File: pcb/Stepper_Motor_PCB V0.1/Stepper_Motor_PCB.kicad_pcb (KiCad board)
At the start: 2 copper layers, 67 x 50.9 mm, 29 parts, among them J1 Pwr/Coms, J2 Pot, J3 Bootloader Pins, J4 Stepper_Motor, J5 LED, J7 8P8C, SW1 SW_Push, U1 ATmega328P-AU, Y1 Crystal

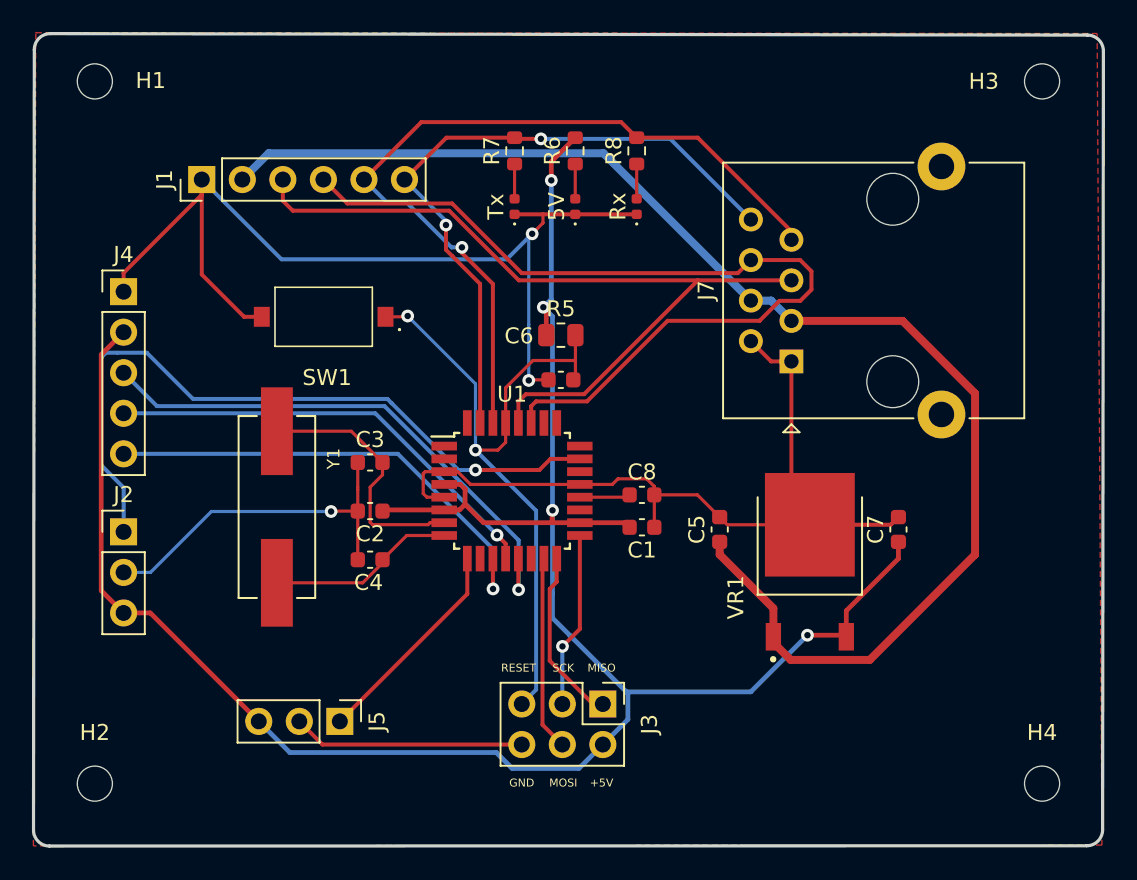
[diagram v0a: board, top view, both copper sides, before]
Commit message: update pcb
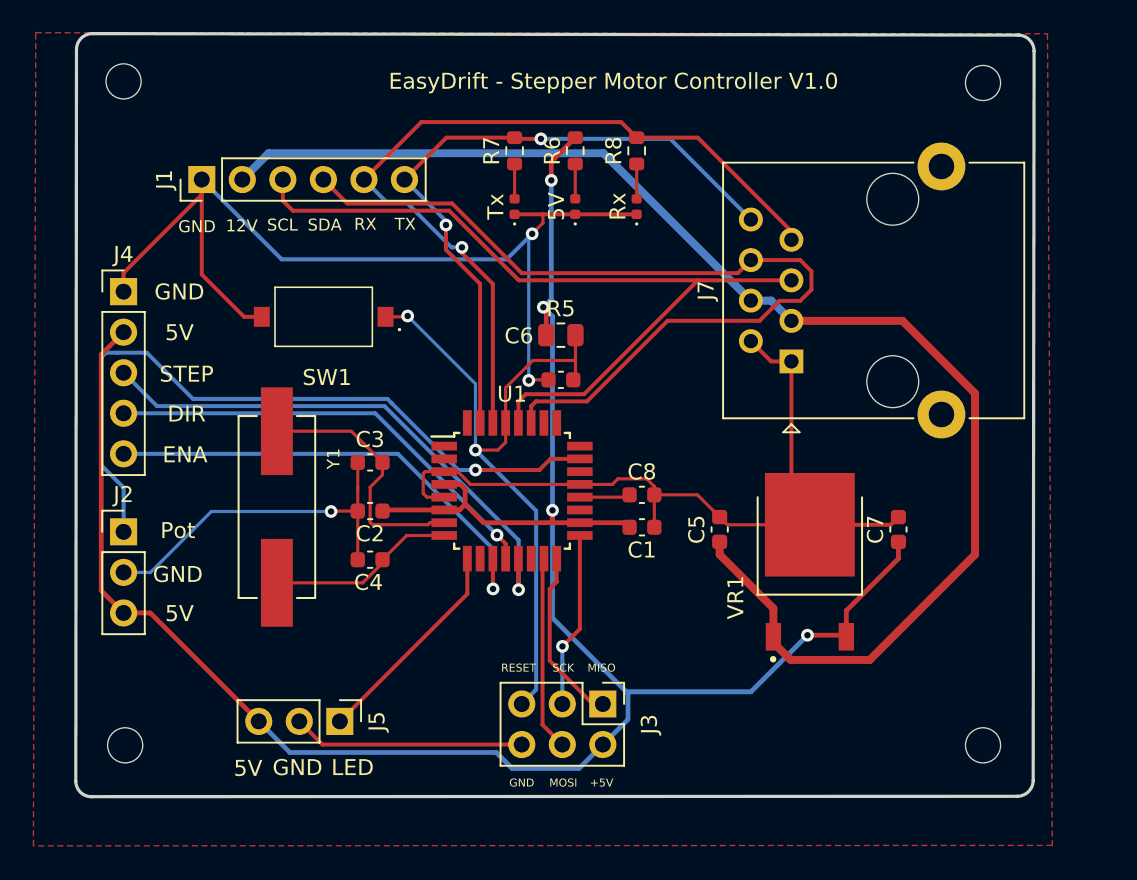
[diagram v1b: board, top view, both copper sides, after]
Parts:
- moved H4 4.41 mm to (178.8, 114.5)
- moved H3 3.70 mm to (178.8, 73.0)
- moved H2 3.06 mm to (125.1, 114.5)
- moved H1 1.80 mm to (125.0, 72.9)
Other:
- board size 67 x 50.9 mm -> 60 x 47.8 mm
- board text added: "12V"
- board text added: "5V"
- board text added: "DIR"
- board text added: "ENA"
- board text added: "EasyDrift - Stepper Motor Controller V1.0"
- board text added: "LED"
- board text added: "Pot"
- board text added: "RX"
- board text added: "SCL"
- board text added: "SDA"
- board text added: "STEP"
- board text added: "TX"
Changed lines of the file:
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@@
   )
   (footprint "MountingHole:MountingHole_2.2mm_M2" (layer "F.Cu")
-    (at 123.2 116.9)
+    (at 125.1 114.5)
     (descr "Mounting Hole 2.2mm, no annular, M2")
     (tags "mounting hole 2.2mm no annular m2")
@@
     (property "Sheetname" "")
     (attr exclude_from_pos_files)
-    (fp_text reference "H2" (at 0 -3.2) (layer "F.SilkS")
+    (fp_text reference "H2" (at 0 -3.2) (layer "F.SilkS") hide
       (effects (font (size 1 1) (thickness 0.15)))
     )
@@
   )
   (footprint "MountingHole:MountingHole_2.2mm_M2" (layer "F.Cu")
-    (at 182.55 72.9)
+    (at 178.85 73)
     (descr "Mounting Hole 2.2mm, no annular, M2")
     (tags "mounting hole 2.2mm no annular m2")
@@
     (property "Sheetname" "")
     (attr exclude_from_pos_files)
-    (fp_text reference "H3" (at -3.65 0) (layer "F.SilkS")
+    (fp_text reference "H3" (at -3.65 0) (layer "F.SilkS") hide
       (effects (font (size 1 1) (thickness 0.15)))
     )
@@
   )
   (footprint "MountingHole:MountingHole_2.2mm_M2" (layer "F.Cu")
-    (at 182.55 116.9)
+    (at 178.85 114.5)
     (descr "Mounting Hole 2.2mm, no annular, M2")
     (tags "mounting hole 2.2mm no annular m2")
@@
     (property "Sheetname" "")
     (attr exclude_from_pos_files)
-    (fp_text reference "H4" (at 0 -3.2) (layer "F.SilkS")
+    (fp_text reference "H4" (at 0 -3.2) (layer "F.SilkS") hide
       (effects (font (size 1 1) (thickness 0.15)))
     )
@@
   )
   (footprint "MountingHole:MountingHole_2.2mm_M2" (layer "F.Cu")
-    (at 123.2 72.9)
+    (at 125 72.9)
     (descr "Mounting Hole 2.2mm, no annular, M2")
     (tags "mounting hole 2.2mm no annular m2")
@@
     (property "Sheetname" "")
     (attr exclude_from_pos_files)
-    (fp_text reference "H1" (at 3.5 -0.05) (layer "F.SilkS")
+    (fp_text reference "H1" (at 3.5 -0.05) (layer "F.SilkS") hide
       (effects (font (size 1 1) (thickness 0.15)))
     )
@@
     )
   )
-  (gr_line (start 185.342893 120.792893) (end 120.357107 120.810661) (layer "Edge.Cuts") (width 0.2))
-  (gr_line (start 119.357107 119.810661) (end 119.407107 70.907107) (layer "Edge.Cuts") (width 0.2))
-  (gr_arc (start 185.392893 70) (mid 186.1 70.292893) (end 186.392893 71) (layer "Edge.Cuts") (width 0.2))
-  (gr_arc (start 119.407107 70.907107) (mid 119.700001 70.200003) (end 120.407107 69.907107) (layer "Edge.Cuts") (width 0.2))
-  (gr_line (start 186.392893 71) (end 186.342893 119.792893) (layer "Edge.Cuts") (width 0.2))
-  (gr_line (start 120.407107 69.907107) (end 185.392893 70) (layer "Edge.Cuts") (width 0.2))
-  (gr_arc (start 120.357107 120.810661) (mid 119.649996 120.51777) (end 119.357107 119.810661) (layer "Edge.Cuts") (width 0.2))
-  (gr_arc (start 186.342893 119.792893) (mid 186.05 120.5) (end 185.342893 120.792893) (layer "Edge.Cuts") (width 0.2))
-  (gr_rect (start 128.257 83.312) (end 160.261 108.966) (layer "User.1") (width 0.5) (fill none))
+  (gr_line (start 180.992893 117.692891) (end 123.007111 117.717768) (layer "Edge.Cuts") (width 0.2))
+  (gr_line (start 122.007111 116.742893) (end 122.05 70.907107) (layer "Edge.Cuts") (width 0.2))
+  (gr_arc (start 181.05 70) (mid 181.757111 70.292891) (end 182.05 71) (layer "Edge.Cuts") (width 0.2))
+  (gr_arc (start 122.05 70.907107) (mid 122.342891 70.199998) (end 123.05 69.907107) (layer "Edge.Cuts") (width 0.2))
+  (gr_line (start 182.05 71) (end 181.992893 116.692891) (layer "Edge.Cuts") (width 0.2))
+  (gr_line (start 123.05 69.907107) (end 181.05 70) (layer "Edge.Cuts") (width 0.2))
+  (gr_arc (start 123.007111 117.717768) (mid 122.301554 117.441185) (end 122.007111 116.742893) (layer "Edge.Cuts") (width 0.2))
+  (gr_arc (start 181.992893 116.692891) (mid 181.700002 117.4) (end 180.992893 117.692891) (layer "Edge.Cuts") (width 0.2))
   (gr_text "MOSI" (at 152.55 116.85) (layer "F.SilkS")
     (effects (font (size 0.5 0.5) (thickness 0.125)))
   )
+  (gr_text "ENA" (at 128.85 96.3) (layer "F.SilkS")
+    (effects (font (size 1 1) (thickness 0.15)))
+  )
+  (gr_text "GND" (at 128.5 86.1) (layer "F.SilkS")
+    (effects (font (size 1 1) (thickness 0.15)))
+  )
   (gr_text "RESET" (at 149.75 109.65) (layer "F.SilkS")
     (effects (font (size 0.5 0.5) (thickness 0.125)))
   )
+  (gr_text "STEP" (at 128.95 91.25) (layer "F.SilkS")
+    (effects (font (size 1 1) (thickness 0.15)))
+  )
   (gr_text "MISO" (at 154.95 109.65) (layer "F.SilkS")
     (effects (font (size 0.5 0.5) (thickness 0.125)))
   )
+  (gr_text "Pot" (at 128.4 101.05) (layer "F.SilkS")
+    (effects (font (size 1 1) (thickness 0.15)))
+  )
+  (gr_text "SDA" (at 137.6 81.9) (layer "F.SilkS")
+    (effects (font (size 0.75 0.75) (thickness 0.15)))
+  )
+  (gr_text "GND" (at 135.9 115.9) (layer "F.SilkS")
+    (effects (font (size 1 1) (thickness 0.15)))
+  )
+  (gr_text "GND" (at 128.4 103.8) (layer "F.SilkS")
+    (effects (font (size 1 1) (thickness 0.15)))
+  )
+  (gr_text "SCL" (at 134.95 81.9) (layer "F.SilkS")
+    (effects (font (size 0.75 0.75) (thickness 0.15)))
+  )
+  (gr_text "EasyDrift - Stepper Motor Controller V1.0" (at 155.7 72.9) (layer "F.SilkS")
+    (effects (font (size 1 1) (thickness 0.15)))
+  )
+  (gr_text "5V" (at 132.8 115.95) (layer "F.SilkS")
+    (effects (font (size 1 1) (thickness 0.15)))
+  )
+  (gr_text "LED" (at 139.35 115.9) (layer "F.SilkS")
+    (effects (font (size 1 1) (thickness 0.15)))
+  )
+  (gr_text "5V" (at 128.5 106.25) (layer "F.SilkS")
+    (effects (font (size 1 1) (thickness 0.15)))
+  )
+  (gr_text "TX" (at 142.65 81.85) (layer "F.SilkS")
+    (effects (font (size 0.75 0.75) (thickness 0.15)))
+  )
+  (gr_text "DIR" (at 128.95 93.75) (layer "F.SilkS")
+    (effects (font (size 1 1) (thickness 0.15)))
+  )
+  (gr_text "12V" (at 132.4 81.95) (layer "F.SilkS")
+    (effects (font (size 0.75 0.75) (thickness 0.15)))
+  )
   (gr_text "SCK" (at 152.55 109.65) (layer "F.SilkS")
     (effects (font (size 0.5 0.5) (thickness 0.125)))
   )
+  (gr_text "5V" (at 128.5 88.65) (layer "F.SilkS")
+    (effects (font (size 1 1) (thickness 0.15)))
+  )
   (gr_text "+5V" (at 154.95 116.85) (layer "F.SilkS")
     (effects (font (size 0.5 0.5) (thickness 0.125)))
+  )
+  (gr_text "GND" (at 129.6 82) (layer "F.SilkS")
+    (effects (font (size 0.75 0.75) (thickness 0.15)))
+  )
+  (gr_text "RX" (at 140.15 81.85) (layer "F.SilkS")
+    (effects (font (size 0.75 0.75) (thickness 0.15)))
   )
   (gr_text "GND" (at 149.95 116.85) (layer "F.SilkS")
@@
       (pts
         (xy 119.5 69.85)
-        (xy 186 69.9)
-        (xy 186.3 120.75)
+        (xy 182.889052 69.918354)
+        (xy 183.189052 120.768354)
         (xy 119.35 120.8)
         (xy 119.5 69.8)
